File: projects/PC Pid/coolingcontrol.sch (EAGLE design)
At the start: 22 parts

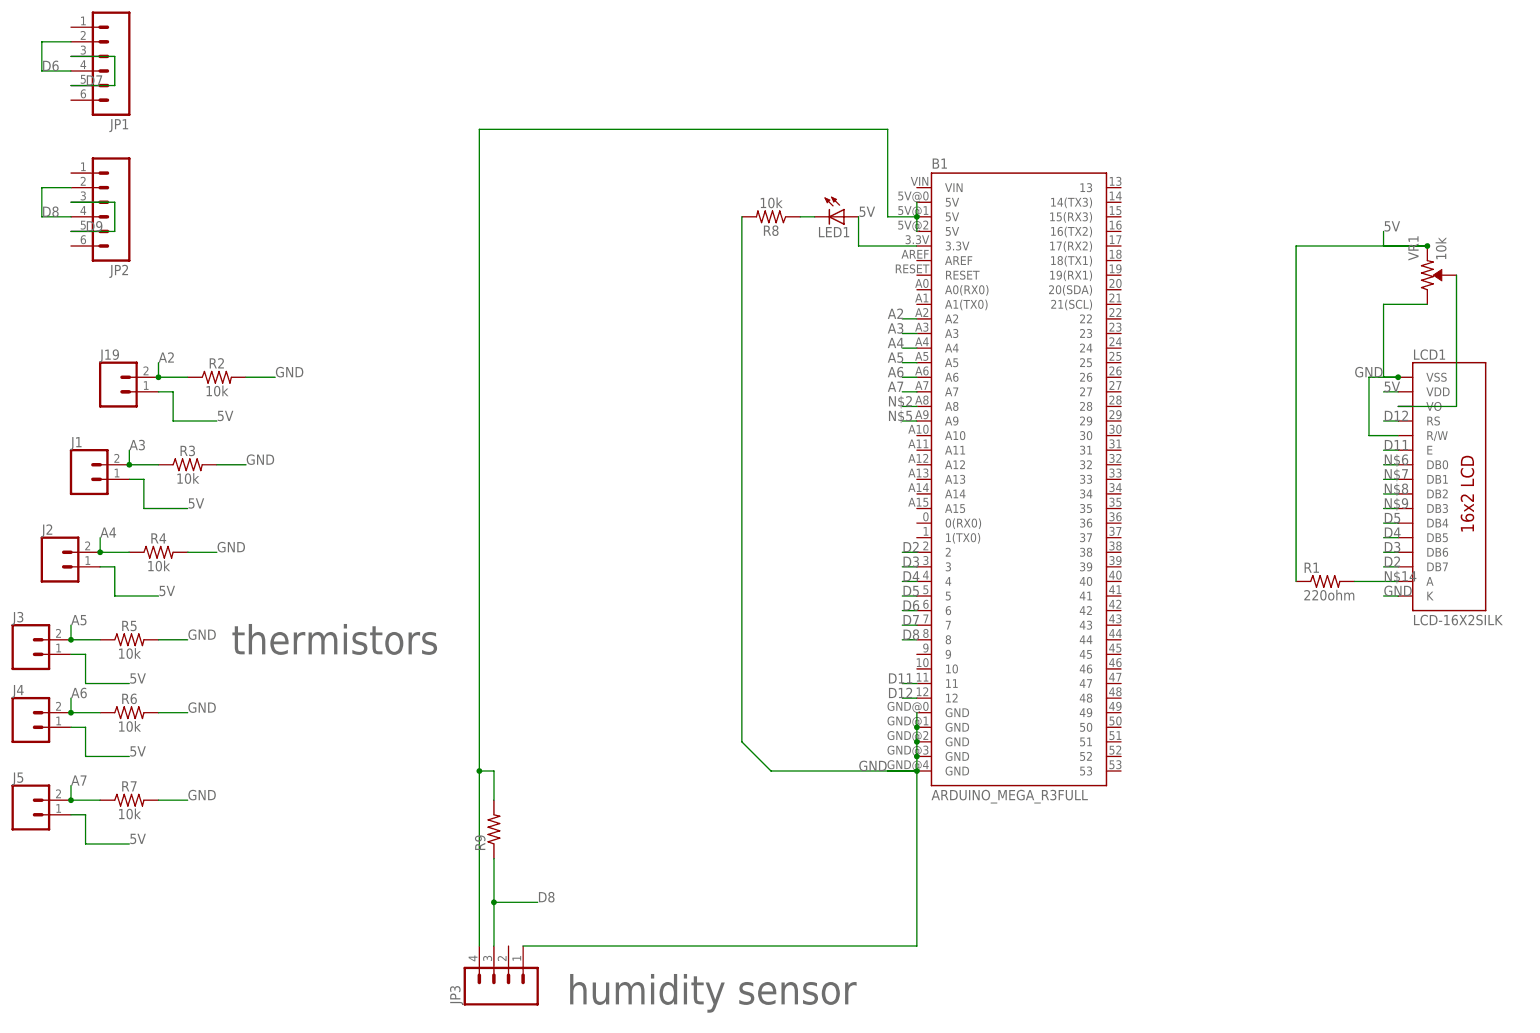
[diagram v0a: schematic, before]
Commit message: asd
asd
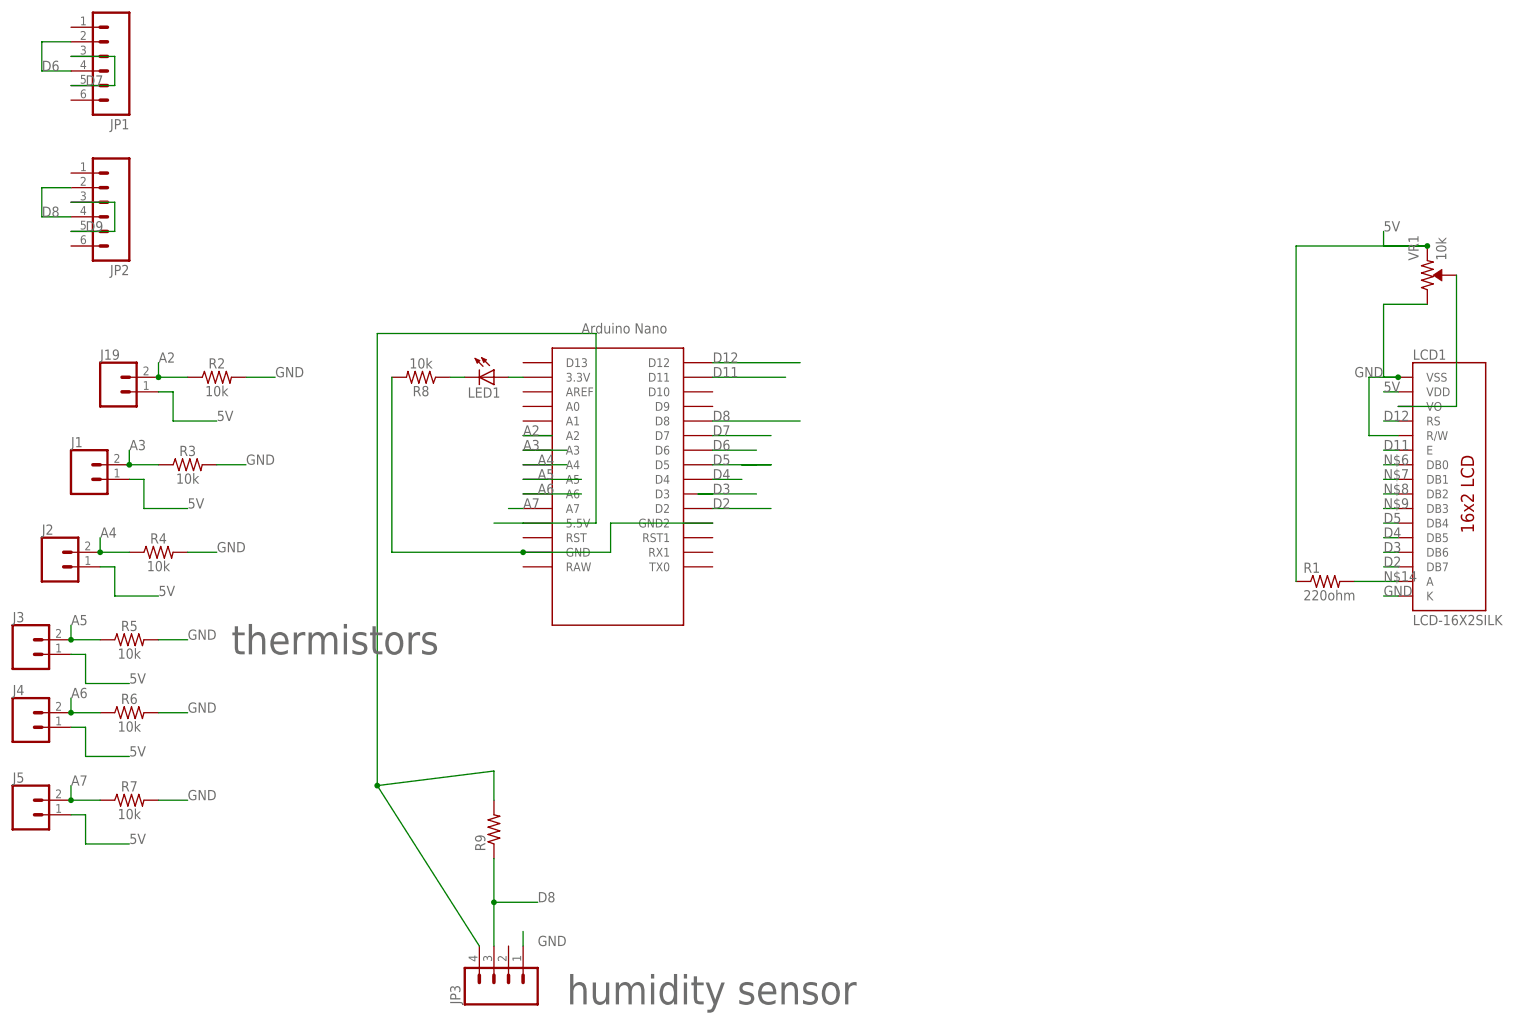
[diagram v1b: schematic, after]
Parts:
- removed B1: ARDUINO_MEGA_R3FULL, SparkFun-Boards:ARDUINO_MEGA_R3FULL
- added U$1: NANO, Arduino-clone:NANO
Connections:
- removed net N$2: B1.A8
- removed net N$5: B1.A9
- net 5V: now also U$1.5.5V; no longer B1.5V@0, B1.5V@1, B1.5V@2
- net A2: now also U$1.A2; no longer B1.A2
- net A3: now also U$1.A3; no longer B1.A3
- net A4: now also U$1.A4; no longer B1.A4
- net A5: now also U$1.A5; no longer B1.A5
- net A6: now also U$1.A6; no longer B1.A6
- net A7: now also U$1.A7; no longer B1.A7
- net D11: now also U$1.D11; no longer B1.11
- net D12: now also U$1.D12; no longer B1.12
- net D2: now also U$1.D2; no longer B1.2
- net D3: now also U$1.D3; no longer B1.3
- net D4: now also U$1.D4; no longer B1.4
- net D5: now also U$1.D5; no longer B1.5
- net D6: now also U$1.D6; no longer B1.6
- net D7: now also U$1.D7; no longer B1.7
- net D8: now also U$1.D8; no longer B1.8
- net GND: now also U$1.GND, U$1.GND2; no longer B1.GND@0, B1.GND@1, B1.GND@2, B1.GND@3, B1.GND@4
- net N$4: now also U$1.3.3V; no longer B1.3.3V
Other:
- moved on the sheet: LED1, R8
